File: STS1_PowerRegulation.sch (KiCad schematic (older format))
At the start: 20 parts, among them U2 LT3120

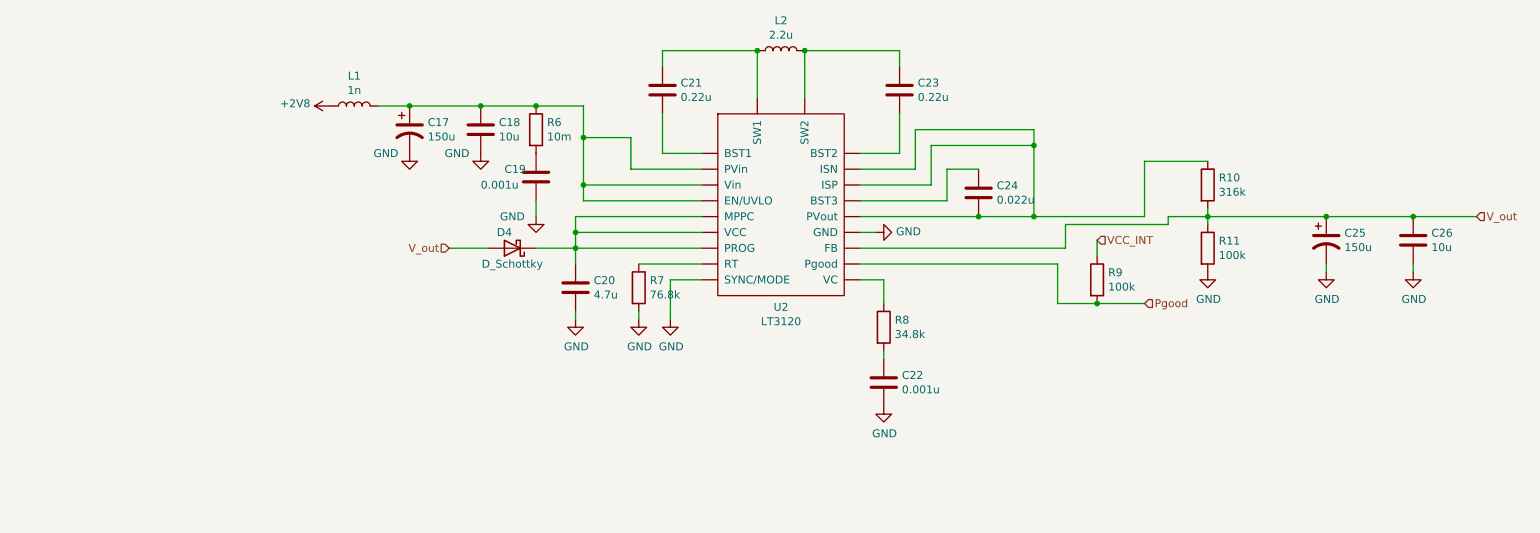
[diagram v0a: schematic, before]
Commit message: schematic done
final tweaks (adding LEDS, pin headers, moving circuits...)
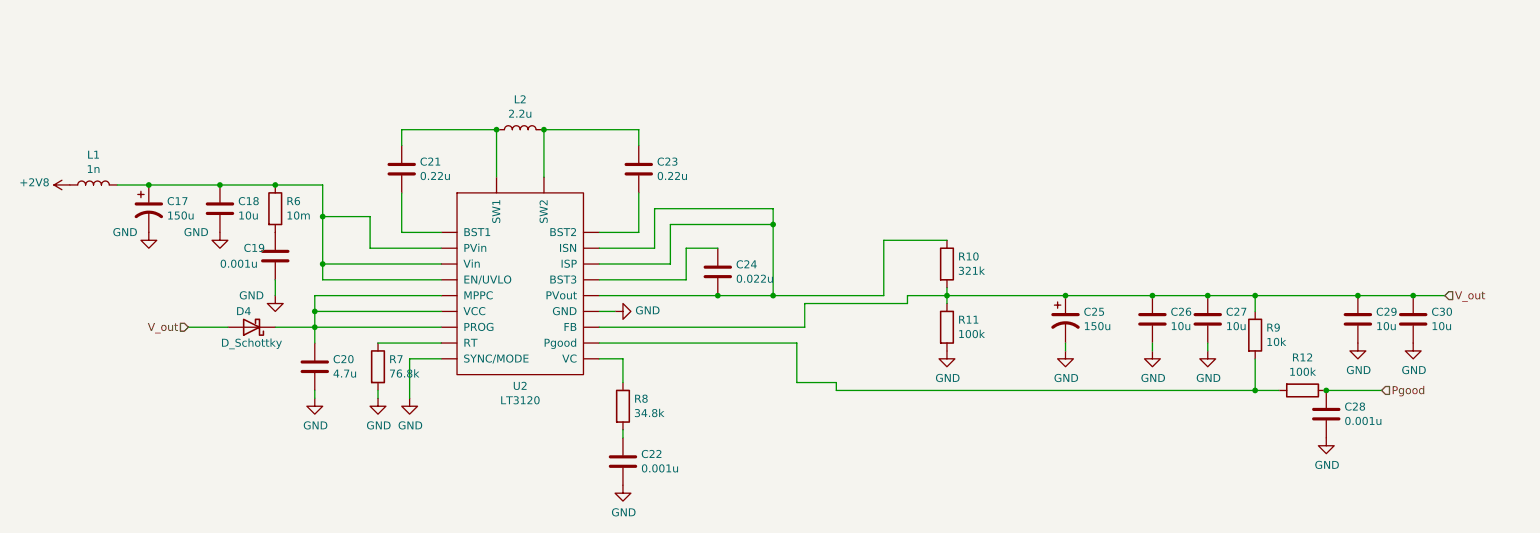
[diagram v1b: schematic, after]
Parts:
- added C27, C29, C30: 10u, symbol Device:C
- added C28: 0.001u, symbol Device:C
- added R12: 100k, symbol Device:R
- R10: value 316k -> 321k
- R9: value 100k -> 10k
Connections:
- net VCC_INT is gone; now on net V_out: R9.1
- net GND: now also C27.2, C28.2, C29.2, C30.2
- net Pgood: now also C28.1, R12.1; no longer R9.2, U2.~ (Vin)
- net V_out: now also C27.1, C29.1, C30.1
- new net: R12.2, R9.2, U2.~ (Vin)
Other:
- moved on the sheet: C17, C18, C19, C20, C21, C22, C23, C24, C25, C26, D4, L1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
